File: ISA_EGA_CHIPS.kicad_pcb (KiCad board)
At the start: 2 copper layers, 131.1 x 108 mm, 67 parts, among them J1 EGA Feature Connector, J2 Light Pen, J3 RCA 1, J4 RCA 2, J6 Digital Output, J7 Bus_ISA_8bit, SW1 Configuration, U1 41464, U10 27C256, U11 82A436, U12 41464, U13 74LS244, U14 41464, U15 74LS244, U2 82C435, U3 41464, U4 74LS244, U5 41464, U6 74LS153, U7 41464, U8 41464, U9 41464

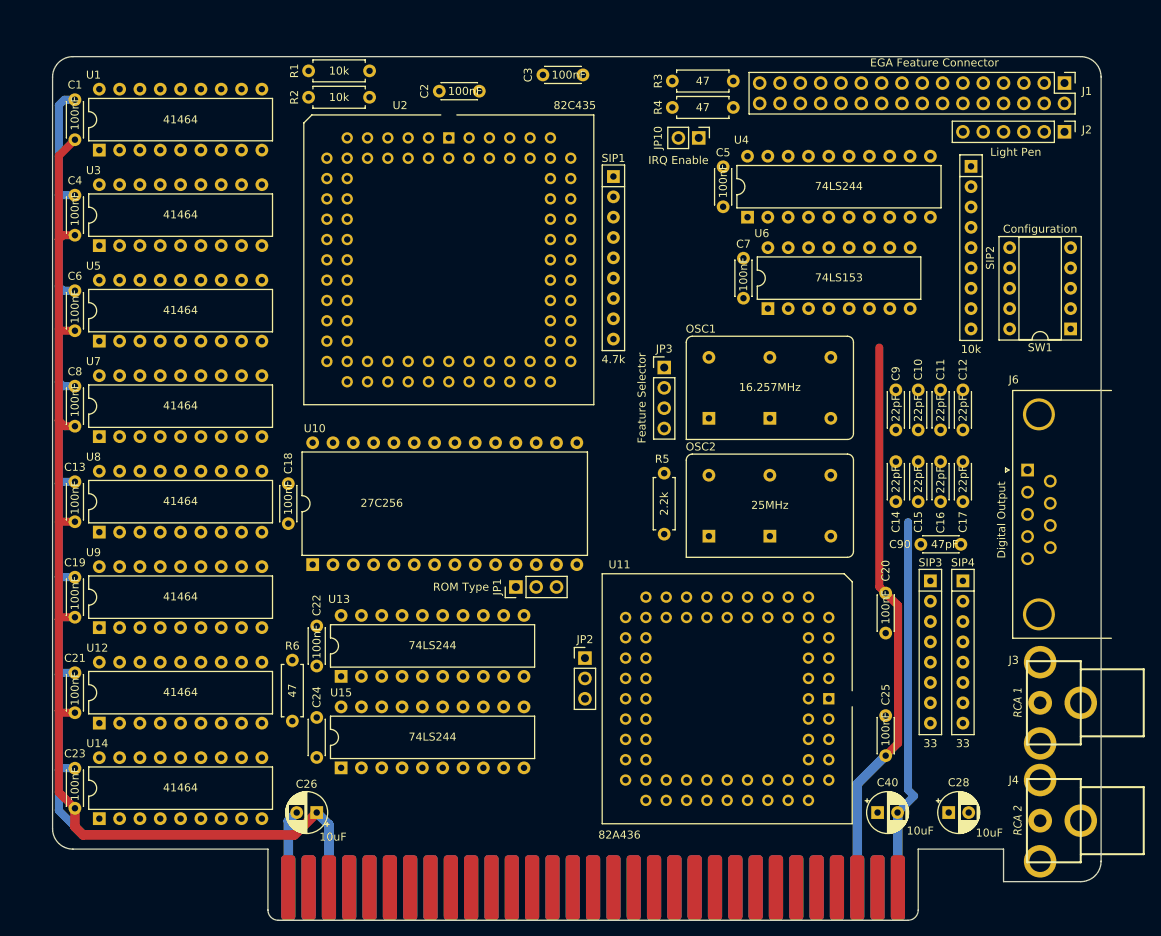
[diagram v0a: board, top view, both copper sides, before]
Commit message: First board render
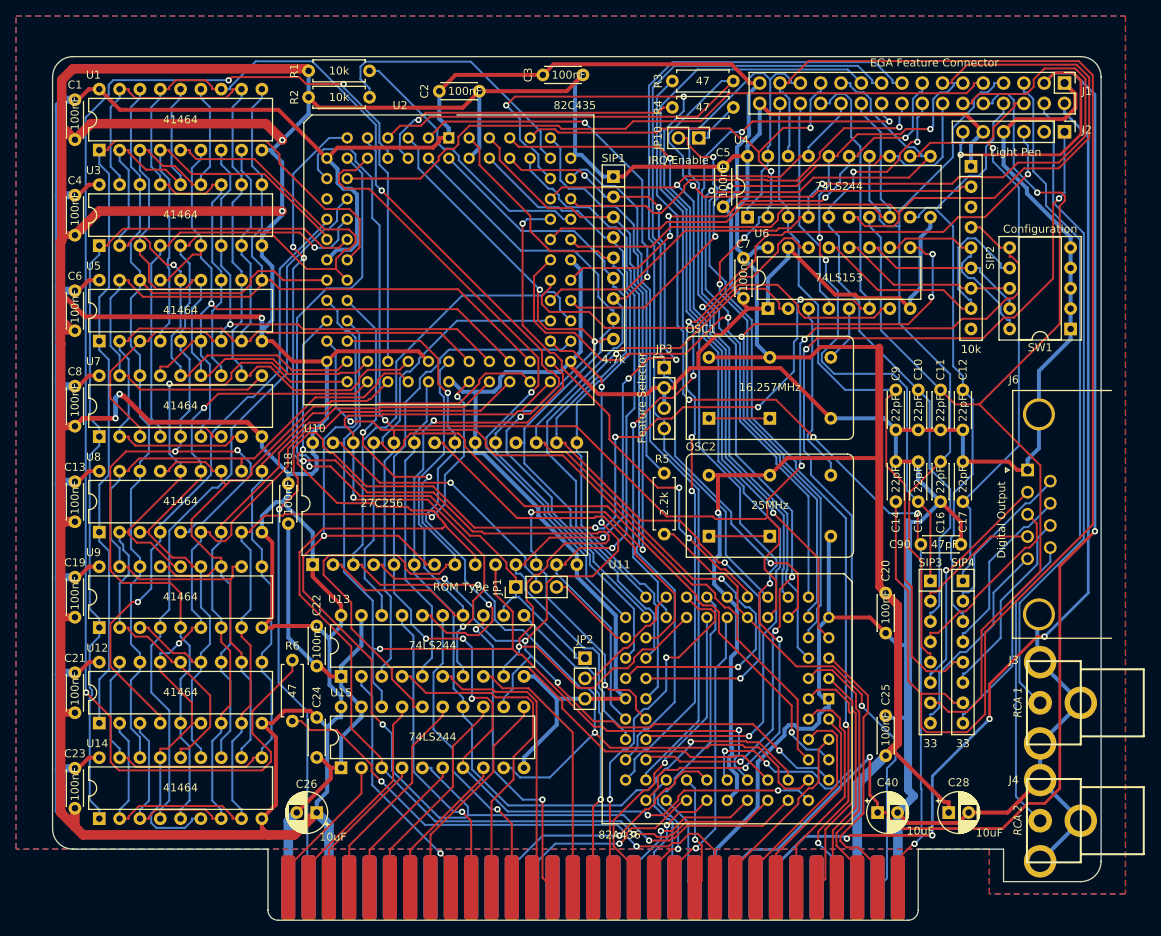
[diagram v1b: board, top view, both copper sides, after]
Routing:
- net GND: track 192.0 -> 863.9 mm
- net VCC: track 213.7 -> 813.6 mm, vias 0 -> 6
- net /BUS_OSC: track 0.00 -> 190.8 mm, vias 0 -> 5
- net +12V: track 0.00 -> 186.3 mm, vias 0 -> 3
- net /BUF_VIN: track 0.00 -> 180.9 mm
- net /IOADS: track 0.00 -> 177.0 mm, vias 0 -> 3
- net /~RAS: track 0.00 -> 169.2 mm, vias 0 -> 2
- net /~IO_RDY: track 0.00 -> 165.5 mm, vias 0 -> 3
- net /BUF_A01: track 0.00 -> 152.2 mm, vias 0 -> 2
- net /BUF_A03: track 0.00 -> 149.0 mm, vias 0 -> 3
- net /BUF_A07: track 0.00 -> 145.1 mm, vias 0 -> 2
- net /LPENSTB: track 0.00 -> 144.1 mm, vias 0 -> 5
- net /BUF_A15: track 0.00 -> 142.6 mm, vias 0 -> 4
- net /BUF_A02: track 0.00 -> 139.5 mm, vias 0 -> 2
- net /BS_V: track 0.00 -> 138.9 mm, vias 0 -> 2
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- added copper zone on B.Cu, net GND
- added copper zone on F.Cu, net GND
